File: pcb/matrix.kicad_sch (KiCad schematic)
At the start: 282 parts

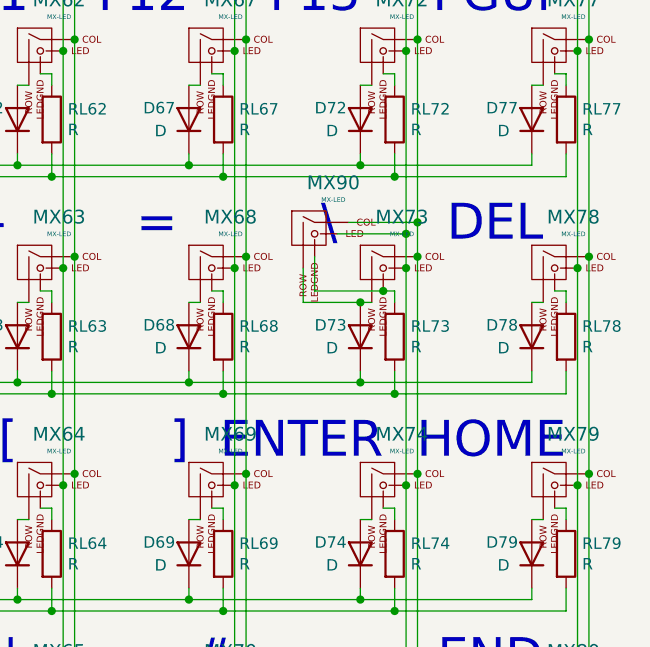
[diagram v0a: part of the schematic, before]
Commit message: added nubs
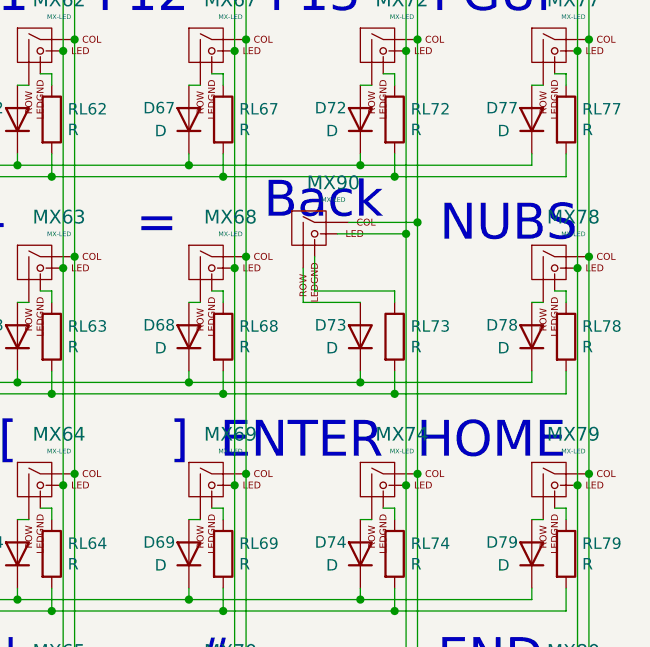
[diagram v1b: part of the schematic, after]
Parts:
- removed MX73: MX-LED, ai03-MX_only:MXOnly-1U, symbol ai03-schematic_library:MX-LED
- MX5: footprint ai03-MX_only:MXOnly-2.25U -> ai03-MX_only:MXOnly-1.25U
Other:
- note added: "Back"
- note added: "NUBS"
- note removed: "DEL"
- note removed: "\"
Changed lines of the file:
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@@
   (junction (at 271.78 113.03) (diameter 0) (color 0 0 0 0)
   )
-  (junction (at 350.52 78.74) (diameter 0) (color 0 0 0 0)
-  )
   (junction (at 220.98 99.06) (diameter 0) (color 0 0 0 0)
   )
@@
   (junction (at 237.49 90.17) (diameter 0) (color 0 0 0 0)
   )
-  (junction (at 354.33 74.93) (diameter 0) (color 0 0 0 0)
-  )
   (junction (at 233.68 137.16) (diameter 0) (color 0 0 0 0)
   )
@@
   (junction (at 200.66 39.37) (diameter 0) (color 0 0 0 0)
   )
-  (junction (at 347.98 80.01) (diameter 0) (color 0 0 0 0)
-  )
   (junction (at 328.93 64.77) (diameter 0) (color 0 0 0 0)
   )
@@
   (junction (at 295.91 39.37) (diameter 0) (color 0 0 0 0)
   )
-  (junction (at 353.06 76.2) (diameter 0) (color 0 0 0 0)
-  )
   (junction (at 238.76 52.07) (diameter 0) (color 0 0 0 0)
   )
@@
     (stroke (width 0) (type default) (color 0 0 0 0))
   )
-  (wire (pts (xy 350.52 78.74) (xy 351.79 78.74))
-    (stroke (width 0) (type default) (color 0 0 0 0))
-  )
   (wire (pts (xy 226.06 243.84) (xy 233.68 243.84))
     (stroke (width 0) (type default) (color 0 0 0 0))
@@
     (stroke (width 0) (type default) (color 0 0 0 0))
   )
-  (wire (pts (xy 354.33 74.93) (xy 354.33 99.06))
+  (wire (pts (xy 354.33 71.12) (xy 354.33 99.06))
     (stroke (width 0) (type default) (color 0 0 0 0))
   )
@@
     (stroke (width 0) (type default) (color 0 0 0 0))
   )
-  (wire (pts (xy 347.98 80.01) (xy 349.25 80.01))
-    (stroke (width 0) (type default) (color 0 0 0 0))
-  )
   (wire (pts (xy 238.76 124.46) (xy 238.76 148.59))
     (stroke (width 0) (type default) (color 0 0 0 0))
@@
     (stroke (width 0) (type default) (color 0 0 0 0))
   )
-  (wire (pts (xy 353.06 72.39) (xy 353.06 76.2))
-    (stroke (width 0) (type default) (color 0 0 0 0))
-  )
   (wire (pts (xy 179.07 261.62) (xy 179.07 269.24))
     (stroke (width 0) (type default) (color 0 0 0 0))
@@
     (stroke (width 0) (type default) (color 0 0 0 0))
   )
-  (wire (pts (xy 342.9 78.74) (xy 350.52 78.74))
+  (wire (pts (xy 342.9 78.74) (xy 351.79 78.74))
     (stroke (width 0) (type default) (color 0 0 0 0))
   )
@@
     (stroke (width 0) (type default) (color 0 0 0 0))
   )
-  (wire (pts (xy 354.33 71.12) (xy 354.33 74.93))
-    (stroke (width 0) (type default) (color 0 0 0 0))
-  )
   (wire (pts (xy 100.33 185.42) (xy 138.43 185.42))
     (stroke (width 0) (type default) (color 0 0 0 0))
@@
     (stroke (width 0) (type default) (color 0 0 0 0))
   )
-  (wire (pts (xy 353.06 76.2) (xy 353.06 100.33))
+  (wire (pts (xy 353.06 72.39) (xy 353.06 100.33))
     (stroke (width 0) (type default) (color 0 0 0 0))
   )
@@
     (stroke (width 0) (type default) (color 0 0 0 0))
   )
-  (text "DEL" (at 368.3 73.66 180)
+  (text "NUBS" (at 372.11 73.66 180)
     (effects (font (size 3.9878 3.9878)) (justify right bottom))
   )
@@
     (effects (font (size 3.9878 3.9878)) (justify right bottom))
   )
-  (text "\\" (at 345.44 73.66 180)
+  (text "Back" (at 350.52 71.12 180)
     (effects (font (size 3.9878 3.9878)) (justify right bottom))
   )
@@
       (effects (font (size 0.508 0.508)))
     )
-    (property "Footprint" "ai03-MX_only:MXOnly-2.25U" (id 2) (at 86.995 149.225 0)
+    (property "Footprint" "ai03-MX_only:MXOnly-1.25U" (id 2) (at 86.995 149.225 0)
       (effects (font (size 1.524 1.524)) hide)
     )
@@
     (pin "2")
   )
-  (symbol (lib_id "ai03-schematic_library:MX-LED") (at 350.52 76.2 0) (unit 1)
-    (in_bom yes) (on_board yes)
-    (property "Reference" "MX73" (id 0) (at 352.6028 70.5358 0)
-      (effects (font (size 1.524 1.524)))
-    )
-    (property "Value" "MX-LED" (id 1) (at 352.6028 72.4154 0)
-      (effects (font (size 0.508 0.508)))
-    )
-    (property "Footprint" "ai03-MX_only:MXOnly-1U" (id 2) (at 334.645 76.835 0)
-      (effects (font (size 1.524 1.524)) hide)
-    )
-    (property "Datasheet" "" (id 3) (at 334.645 76.835 0)
-      (effects (font (size 1.524 1.524)) hide)
-    )
-    (pin "1")
-    (pin "2")
-    (pin "3")
-    (pin "4")
-  )
   (symbol (lib_id "ai03-schematic_library:MX-LED") (at 217.17 76.2 0) (unit 1)
